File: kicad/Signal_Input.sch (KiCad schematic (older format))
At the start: 30 parts, among them J2 CONN_COAXIAL, J3 CONN_COAXIAL, J4 CONN_COAXIAL, T1 WBC16-1T, U10 MC12093, U12 TLV3501, U13 ADR5040, U9 LTC6957-3

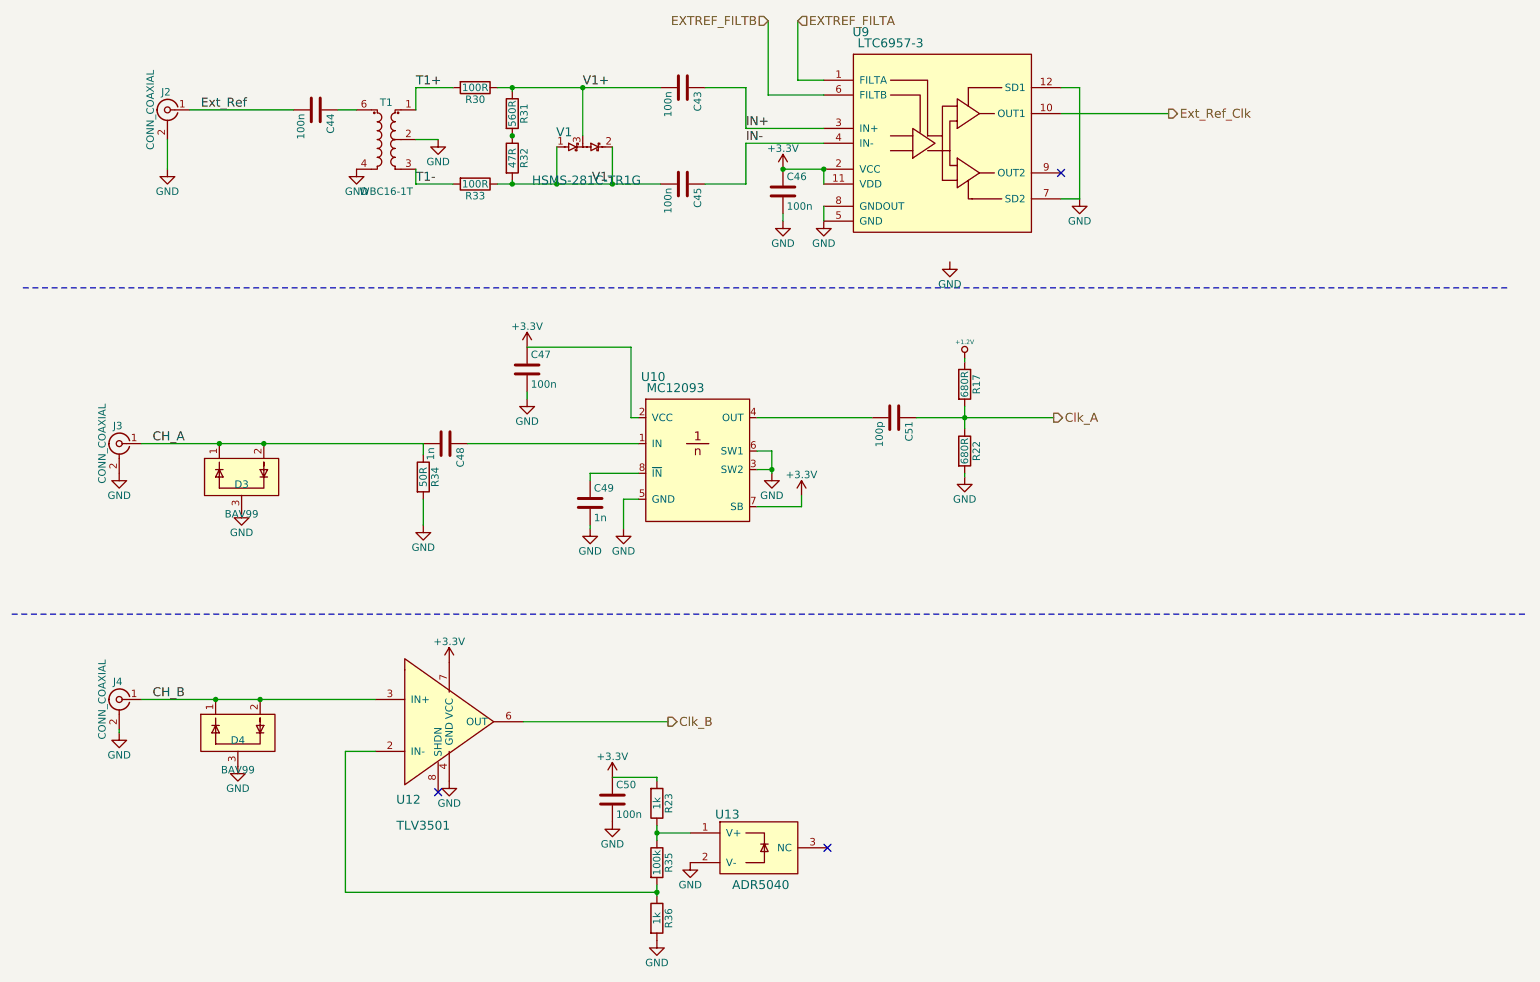
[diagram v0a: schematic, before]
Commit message: some small schematic and layout changes [completed]
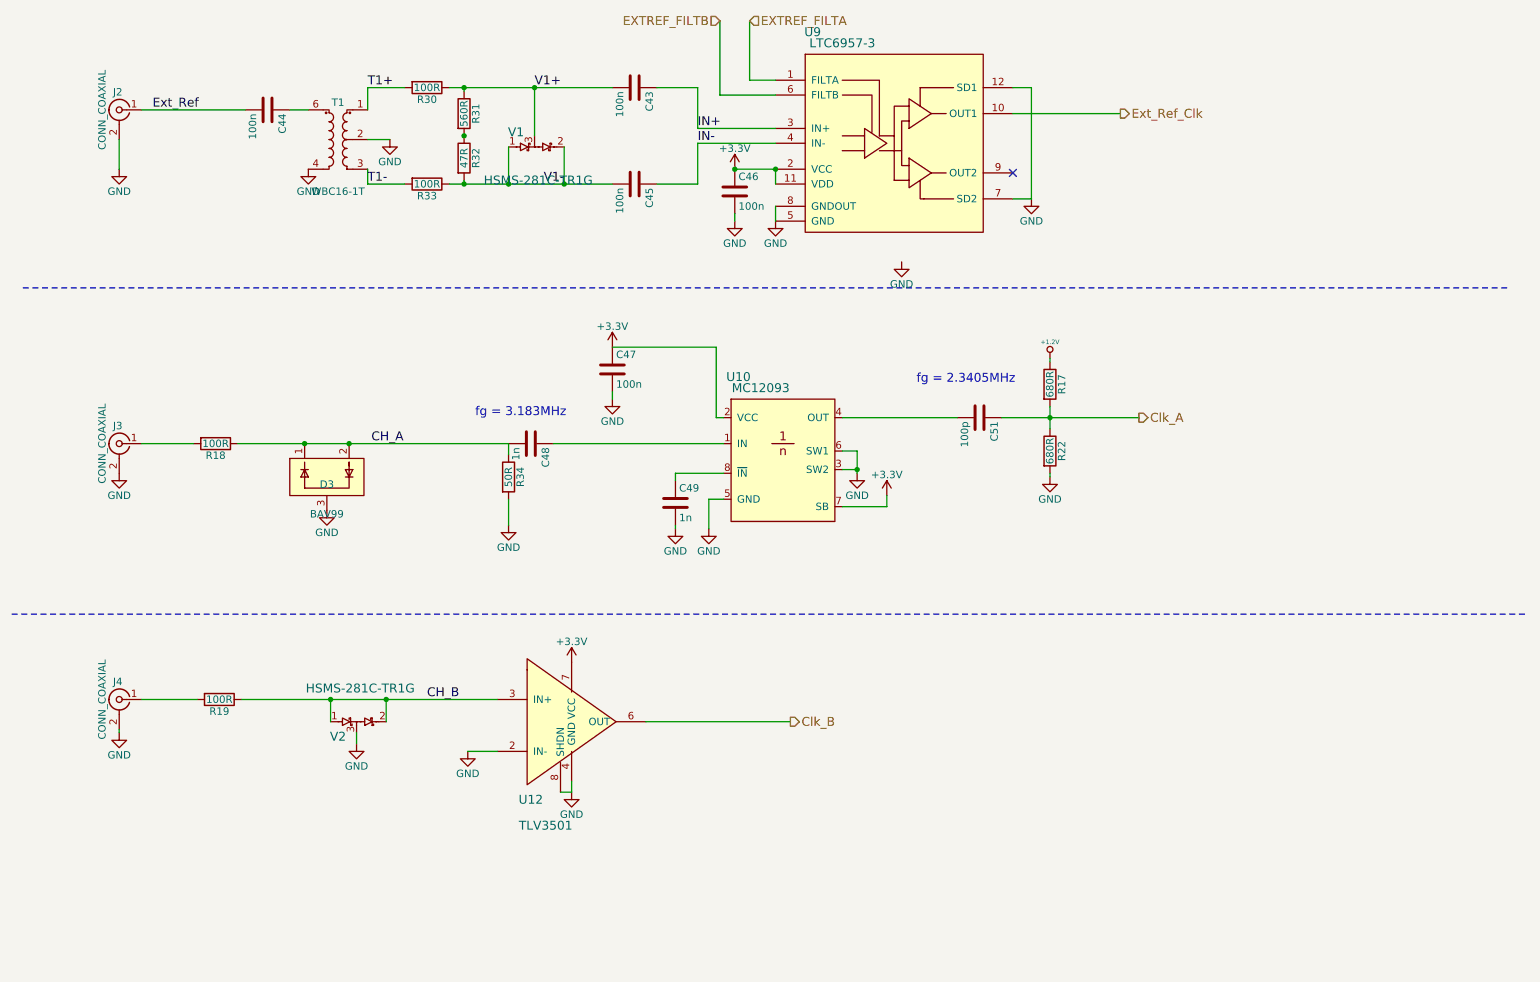
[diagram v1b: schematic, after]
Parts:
- removed C50: 100n, Capacitors_SMD:C_0603_HandSoldering, symbol C
- removed D4: BAV99, TO_SOT_Packages_SMD:SOT-23, symbol BAV99
- removed R23, R36: 1k, Resistors_SMD:R_0603_HandSoldering, symbol R
- removed R35: 100k, Resistors_SMD:R_0603_HandSoldering, symbol R
- removed U13: ADR5040, TO_SOT_Packages_SMD:SOT-323_SC-70_Handsoldering, symbol ADR5040
- added R18, R19: 100R, Resistors_SMD:R_0603_HandSoldering, symbol R
- added V2: HSMS-281C-TR1G, TO_SOT_Packages_SMD:SOT-323_SC-70_Handsoldering, symbol HSMS-281C-TR1G
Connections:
- net CH_A: now also R18.1; no longer J3.1 (In)
- net CH_B: now also R19.1, V2.1, V2.2; no longer J4.1 (In)
- net GND: now also U12.2 (IN-), U12.8 (SHDN), V2.3
- new net: J3.1 (In), R18.2
- new net: J4.1 (In), R19.2
- no-connect marks 3 -> 1
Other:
- note added: "fg = 2.3405MHz\n"
- note added: "fg = 3.183MHz\n"
- moved on the sheet: C43, C44, C45, C46, C47, C48, C49, C51, D3, J2, R17, R22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
